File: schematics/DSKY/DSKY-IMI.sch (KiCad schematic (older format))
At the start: 7 parts, among them J103 Conn_02x08, J104 Conn_02x10, U201 74LS32, U42 74LS04, U46 74LS04, U5 74LS04, U6 74LS00

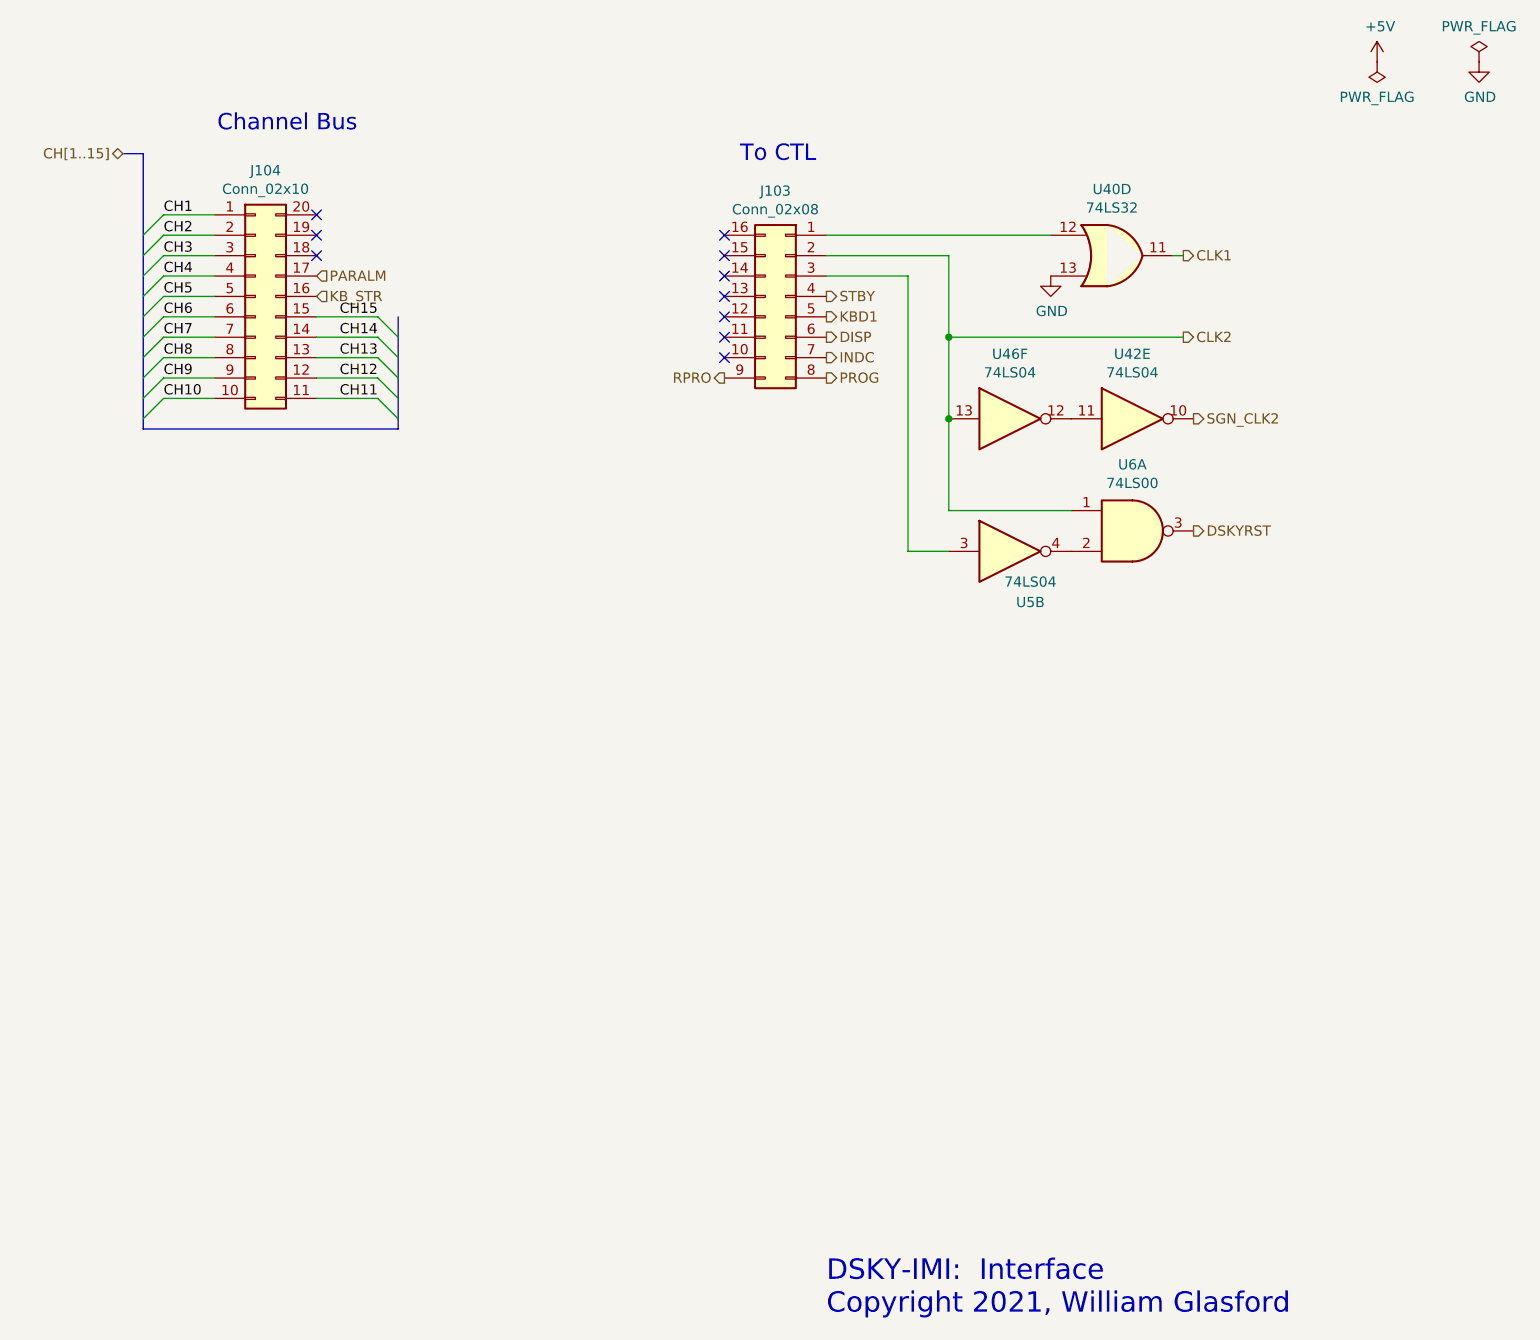
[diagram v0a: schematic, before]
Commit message: Final tweaks, the DSKY is now complete!
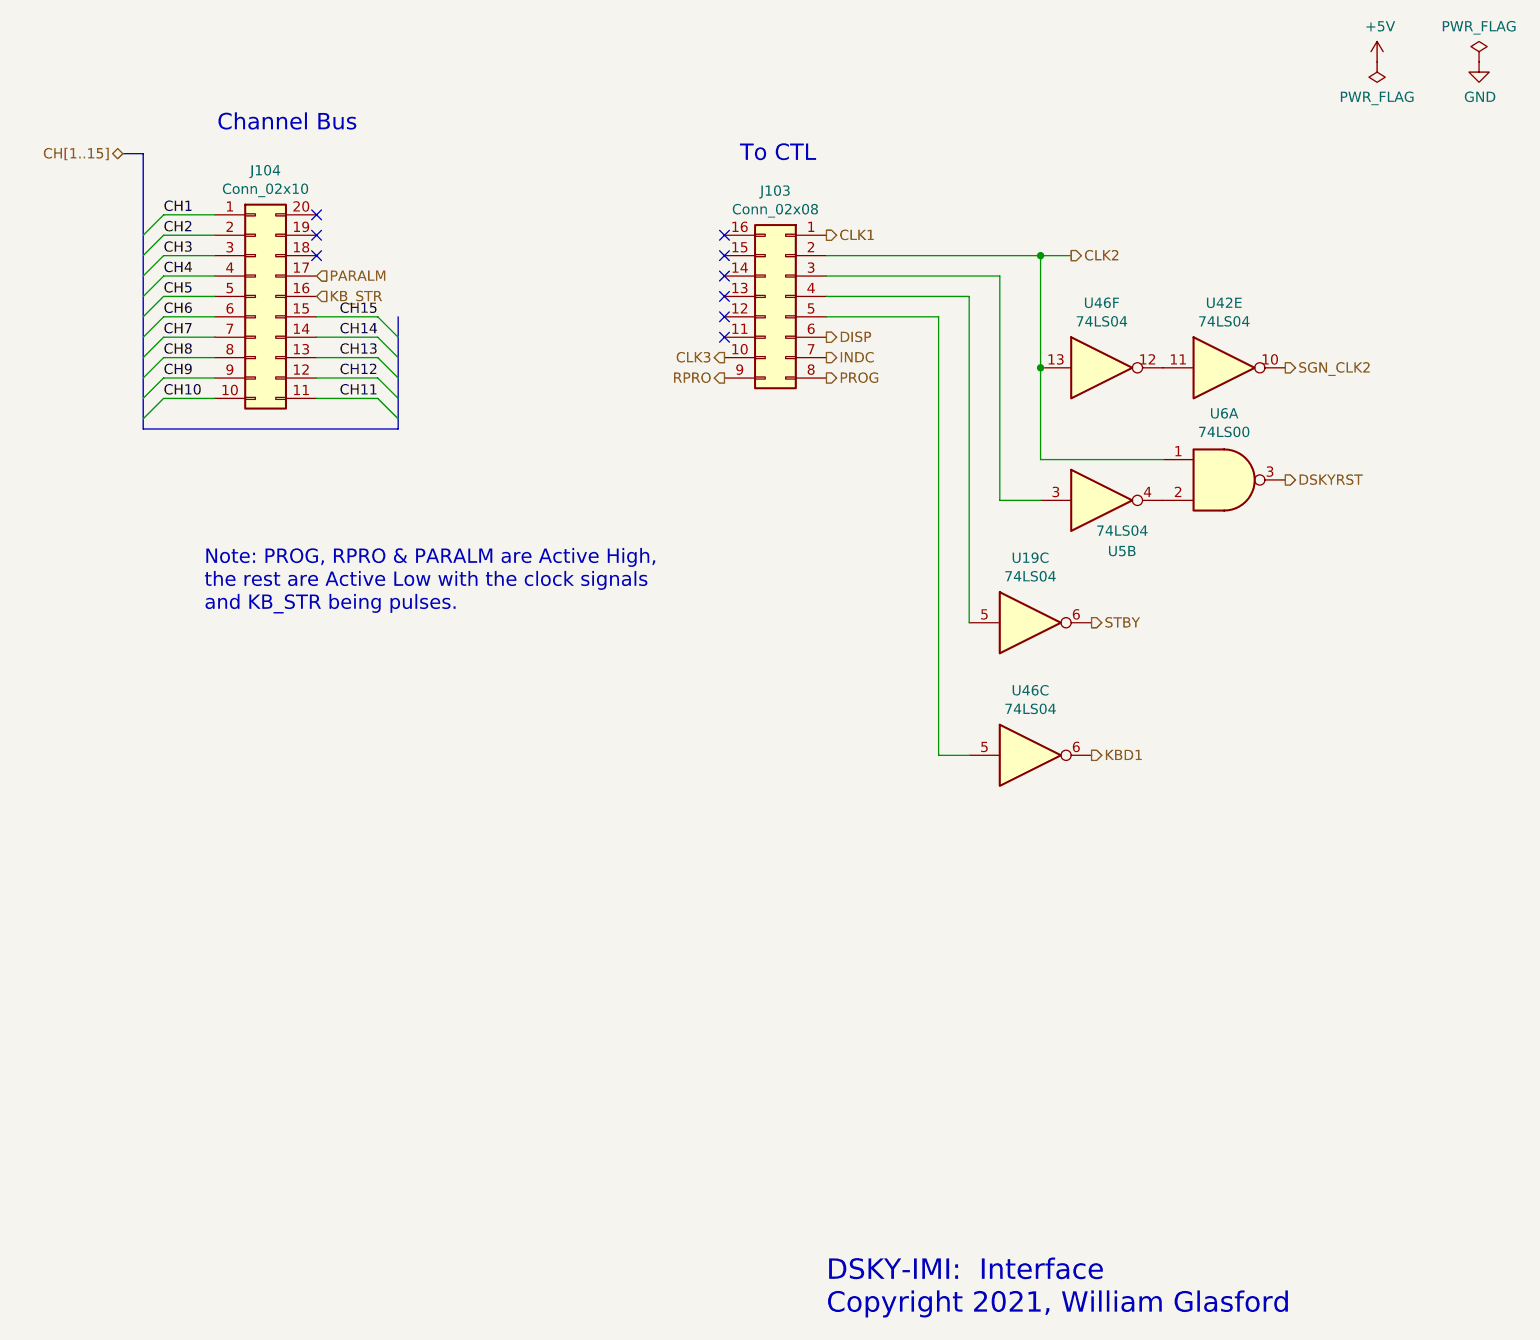
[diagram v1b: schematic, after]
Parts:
- removed U201: 74LS32, symbol 74xx:74LS32
- added U19: 74LS04, symbol 74xx:74LS04
- added unit 3 of U46
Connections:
- net CLK1: now also J103.1 (Pin_1)
- net KBD1: now also U46.6; no longer J103.5 (Pin_5)
- net STBY: now also U19.6; no longer J103.4 (Pin_4)
- net CLK3: now reaches J103.10 (Pin_10)
- new net: J103.4 (Pin_4), U19.5
- new net: J103.5 (Pin_5), U46.5
- no-connect marks 10 -> 9
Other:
- note added: "Note: PROG, RPRO & PARALM are Active High,\nthe rest are Active Low with the clock signals\nand KB_STR being pulses."
- moved on the sheet: U42E, U46F, U5B, U6A
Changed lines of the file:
@@
 Comment4 ""
 $EndDescr
-$Comp
-L power:GND #PWR0102
-U 1 1 5F61EFB4
-P 7500 2050
-AR Path="/5F5E4E3B/5F5F82D4/5F61EFB4" Ref="#PWR0102"  Part="1"
-AR Path="/60F989FD/5F61EFB4" Ref="#PWR0102"  Part="1"
-F 0 "#PWR0102" H 7500 1800 50  0001 C CNN
-F 1 "GND" H 7505 1877 50  0000 C CNN
-F 2 "" H 7500 2050 50  0001 C CNN
-F 3 "" H 7500 2050 50  0001 C CNN
-	1    7500 2050
-	1    0    0    -1
-$EndComp
-Wire Wire Line
-	8150 1950 8100 1950
-Text HLabel 8150 2350 2    50   Output ~ 0
+Text HLabel 7600 1950 2    50   Output ~ 0
 CLK2
-Text HLabel 8150 1950 2    50   Output ~ 0
+Text HLabel 6400 1850 2    50   Output ~ 0
 CLK1
 Wire Wire Line
@@
 Wire Wire Line
 	3900 2250 4200 2250
-Text HLabel 6400 2150 2    50   Output ~ 0
+Text HLabel 7700 3750 2    50   Output ~ 0
 STBY
 Text HLabel 3900 2150 2    50   Input ~ 0
@@
 Text Notes 6350 1500 2    80   ~ 0
 To CTL
-Text HLabel 6400 2250 2    50   Output ~ 0
+Text HLabel 7700 4400 2    50   Output ~ 0
 KBD1
 Text HLabel 6400 2350 2    50   Output ~ 0
@@
 INDC
 NoConn ~ 5900 2350
-NoConn ~ 5900 2450
-Wire Wire Line
-	6400 1850 7500 1850
 Wire Bus Line
 	4300 2800 3050 2800
-$Comp
-L 74xx:74LS32 U201
-U 4 1 5F6065A8
-P 7800 1950
-AR Path="/5F5E4E3B/5F5F82D4/5F6065A8" Ref="U201"  Part="1"
-AR Path="/60F989FD/5F6065A8" Ref="U40"  Part="4"
-F 0 "U40" H 7800 2275 50  0000 C CNN
-F 1 "74LS32" H 7800 2184 50  0000 C CNN
-F 2 "" H 7800 1950 50  0001 C CNN
-F 3 "http://www.ti.com/lit/gpn/sn74LS32" H 7800 1950 50  0001 C CNN
-	4    7800 1950
-	1    0    0    -1
-$EndComp
 Text Notes 6400 7150 0    100  ~ 0
 DSKY-IMI:  Interface\nCopyright 2021, William Glasford
@@
 Text HLabel 5900 2550 0    50   Output ~ 0
 RPRO
-Text HLabel 8200 3300 2    50   Output ~ 0
+Text HLabel 8650 3050 2    50   Output ~ 0
 DSKYRST
 $Comp
 L 74xx:74LS00 U?
 U 1 1 6395652F
-P 7900 3300
+P 8350 3050
 AR Path="/5F5E4E3B/5F5F8347/6395652F" Ref="U?"  Part="1"
 AR Path="/60F98A72/6395652F" Ref="U?"  Part="1"
@@
 AR Path="/60F98A72/66CE2F9E/6395652F" Ref="U?"  Part="1"
 AR Path="/60F989FD/6395652F" Ref="U6"  Part="1"
-F 0 "U6" H 7900 3625 50  0000 C CNN
-F 1 "74LS00" H 7900 3534 50  0000 C CNN
-F 2 "" H 7900 3300 50  0001 C CNN
-F 3 "http://www.ti.com/lit/gpn/sn74ls00" H 7900 3300 50  0001 C CNN
-	1    7900 3300
+F 0 "U6" H 8350 3375 50  0000 C CNN
+F 1 "74LS00" H 8350 3284 50  0000 C CNN
+F 2 "" H 8350 3050 50  0001 C CNN
+F 3 "http://www.ti.com/lit/gpn/sn74ls00" H 8350 3050 50  0001 C CNN
+	1    8350 3050
 	1    0    0    -1
 $EndComp
@@
 L 74xx:74LS04 U?
 U 2 1 63956535
-P 7300 3400
+P 7750 3150
 AR Path="/5F5E4E3B/5F5F8347/63956535" Ref="U?"  Part="6"
 AR Path="/60F98A72/63956535" Ref="U?"  Part="2"
@@
 AR Path="/60F98A72/66CE2F9E/63956535" Ref="U?"  Part="6"
 AR Path="/60F989FD/63956535" Ref="U5"  Part="2"
-F 0 "U5" H 7400 3150 50  0000 C CNN
-F 1 "74LS04" H 7400 3250 50  0000 C CNN
-F 2 "" H 7300 3400 50  0001 C CNN
-F 3 "http://www.ti.com/lit/gpn/sn74LS04" H 7300 3400 50  0001 C CNN
-	2    7300 3400
-	1    0    0    -1
-$EndComp
-Wire Wire Line
-	6400 2050 6800 2050
-Wire Wire Line
-	6800 2050 6800 3400
-Wire Wire Line
-	6800 3400 7000 3400
+F 0 "U5" H 7850 2900 50  0000 C CNN
+F 1 "74LS04" H 7850 3000 50  0000 C CNN
+F 2 "" H 7750 3150 50  0001 C CNN
+F 3 "http://www.ti.com/lit/gpn/sn74LS04" H 7750 3150 50  0001 C CNN
+	2    7750 3150
+	1    0    0    -1
+$EndComp
+Wire Wire Line
+	6400 2050 7250 2050
+Wire Wire Line
+	7250 2050 7250 3150
+Wire Wire Line
+	7250 3150 7450 3150
 $Comp
 L 74xx:74LS04 U42
 U 5 1 6247150B
-P 7900 2750
-F 0 "U42" H 7900 3067 50  0000 C CNN
-F 1 "74LS04" H 7900 2976 50  0000 C CNN
-F 2 "" H 7900 2750 50  0001 C CNN
-F 3 "http://www.ti.com/lit/gpn/sn74LS04" H 7900 2750 50  0001 C CNN
-	5    7900 2750
+P 8350 2500
+F 0 "U42" H 8350 2817 50  0000 C CNN
+F 1 "74LS04" H 8350 2726 50  0000 C CNN
+F 2 "" H 8350 2500 50  0001 C CNN
+F 3 "http://www.ti.com/lit/gpn/sn74LS04" H 8350 2500 50  0001 C CNN
+	5    8350 2500
 	1    0    0    -1
 $EndComp
@@
 L 74xx:74LS04 U46
 U 6 1 62471E0E
-P 7300 2750
-F 0 "U46" H 7300 3067 50  0000 C CNN
-F 1 "74LS04" H 7300 2976 50  0000 C CNN
-F 2 "" H 7300 2750 50  0001 C CNN
-F 3 "http://www.ti.com/lit/gpn/sn74LS04" H 7300 2750 50  0001 C CNN
-	6    7300 2750
-	1    0    0    -1
-$EndComp
-Wire Wire Line
-	6400 1950 7000 1950
-Wire Wire Line
-	7000 1950 7000 2350
-Wire Wire Line
-	8150 2350 7000 2350
-Connection ~ 7000 2350
-Wire Wire Line
-	7000 2350 7000 2750
-Wire Wire Line
-	7000 2750 7000 3200
-Wire Wire Line
-	7000 3200 7600 3200
-Connection ~ 7000 2750
-Text HLabel 8200 2750 2    50   Output ~ 0
+P 7750 2500
+F 0 "U46" H 7750 2817 50  0000 C CNN
+F 1 "74LS04" H 7750 2726 50  0000 C CNN
+F 2 "" H 7750 2500 50  0001 C CNN
+F 3 "http://www.ti.com/lit/gpn/sn74LS04" H 7750 2500 50  0001 C CNN
+	6    7750 2500
+	1    0    0    -1
+$EndComp
+Wire Wire Line
+	6400 1950 7450 1950
+Wire Wire Line
+	7600 1950 7450 1950
+Wire Wire Line
+	7450 2950 8050 2950
+Text HLabel 8650 2500 2    50   Output ~ 0
 SGN_CLK2
+Wire Wire Line
+	7450 1950 7450 2500
+Connection ~ 7450 1950
+Connection ~ 7450 2500
+Wire Wire Line
+	7450 2500 7450 2950
+Text Notes 3350 3700 0    70   ~ 0
+Note: PROG, RPRO & PARALM are Active High,\nthe rest are Active Low with the clock signals\nand KB_STR being pulses.
+$Comp
+L 74xx:74LS04 U19
+U 3 1 61EE72FE
+P 7400 3750
+F 0 "U19" H 7400 4067 50  0000 C CNN
+F 1 "74LS04" H 7400 3976 50  0000 C CNN
+F 2 "" H 7400 3750 50  0001 C CNN
+F 3 "http://www.ti.com/lit/gpn/sn74LS04" H 7400 3750 50  0001 C CNN
+	3    7400 3750
+	1    0    0    -1
+$EndComp
+Wire Wire Line
+	6400 2150 7100 2150
+Wire Wire Line
+	7100 2150 7100 3750
+$Comp
+L 74xx:74LS04 U46
+U 3 1 61F122AA
+P 7400 4400
+F 0 "U46" H 7400 4717 50  0000 C CNN
+F 1 "74LS04" H 7400 4626 50  0000 C CNN
+F 2 "" H 7400 4400 50  0001 C CNN
+F 3 "http://www.ti.com/lit/gpn/sn74LS04" H 7400 4400 50  0001 C CNN
+	3    7400 4400
+	1    0    0    -1
+$EndComp
+Wire Wire Line
+	6400 2250 6950 2250
+Wire Wire Line
+	6950 2250 6950 4400
+Wire Wire Line
+	6950 4400 7100 4400
 Wire Bus Line
 	4300 2250 4300 2800
 Wire Bus Line
 	3050 1450 3050 2800
+Text HLabel 5900 2450 0    50   Output ~ 0
+CLK3
 $EndSCHEMATC
